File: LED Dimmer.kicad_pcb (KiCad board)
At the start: 2 copper layers, 118.1 x 74.9 mm, 82 parts, among them P1 Red Load, P2 Green Load, P3 Blue Load, P4 PWR, Q1 TIP31C, Q2 TIP31C, Q3 TIP31C, Q4 Q_PNP_EBC, Q5 Q_PNP_EBC, Q6 Q_NPN_EBC, SW1 SW_SPDT, SW10 SW_SPDT, SW11 SW_SPDT, SW12 SW_SPDT, SW2 SW_SPDT, SW3 SW_SPDT, SW4 SW_SPDT, SW5 SW_SPDT, SW6 SW_SPDT, SW7 SW_SPDT, SW8 SW_SPDT, SW9 SW_SPDT, U1 LM358, U2 LM358, U3 LM358, U4 LM555N

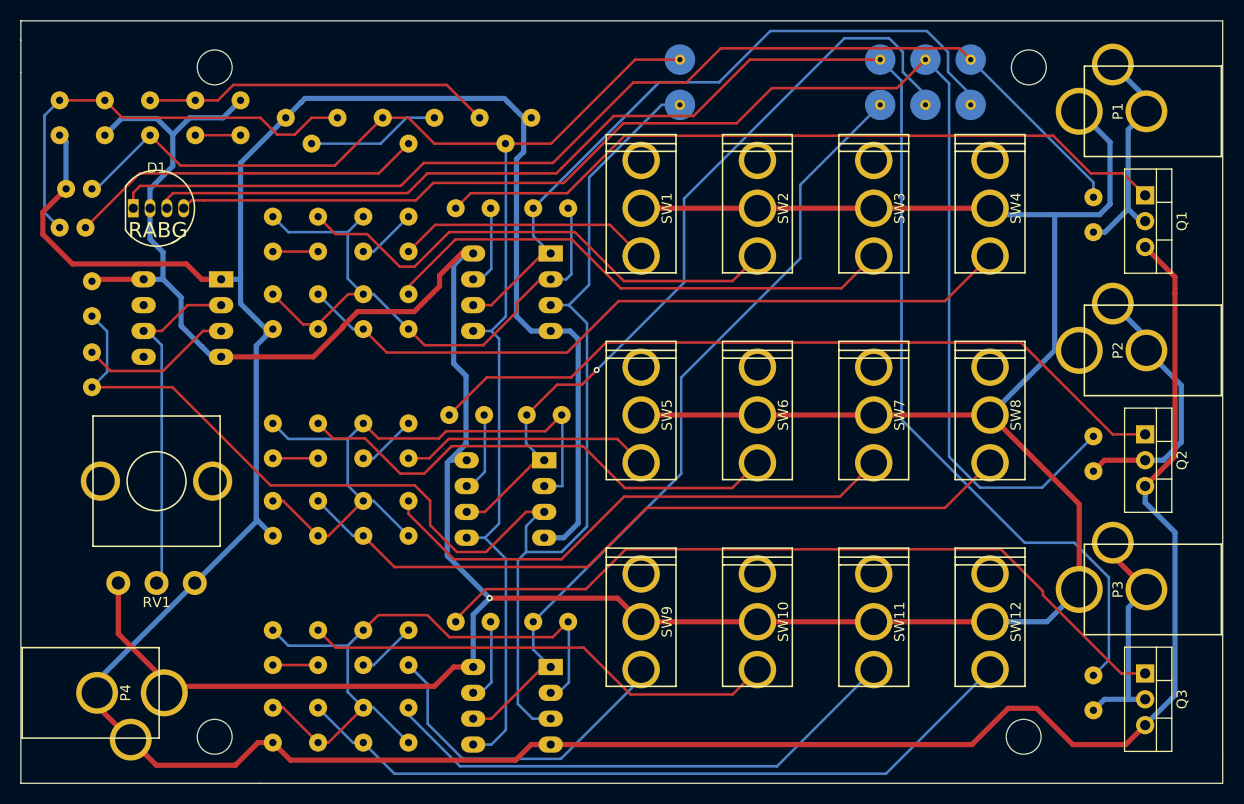
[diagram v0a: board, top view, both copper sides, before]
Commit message: Copper pour, maybe
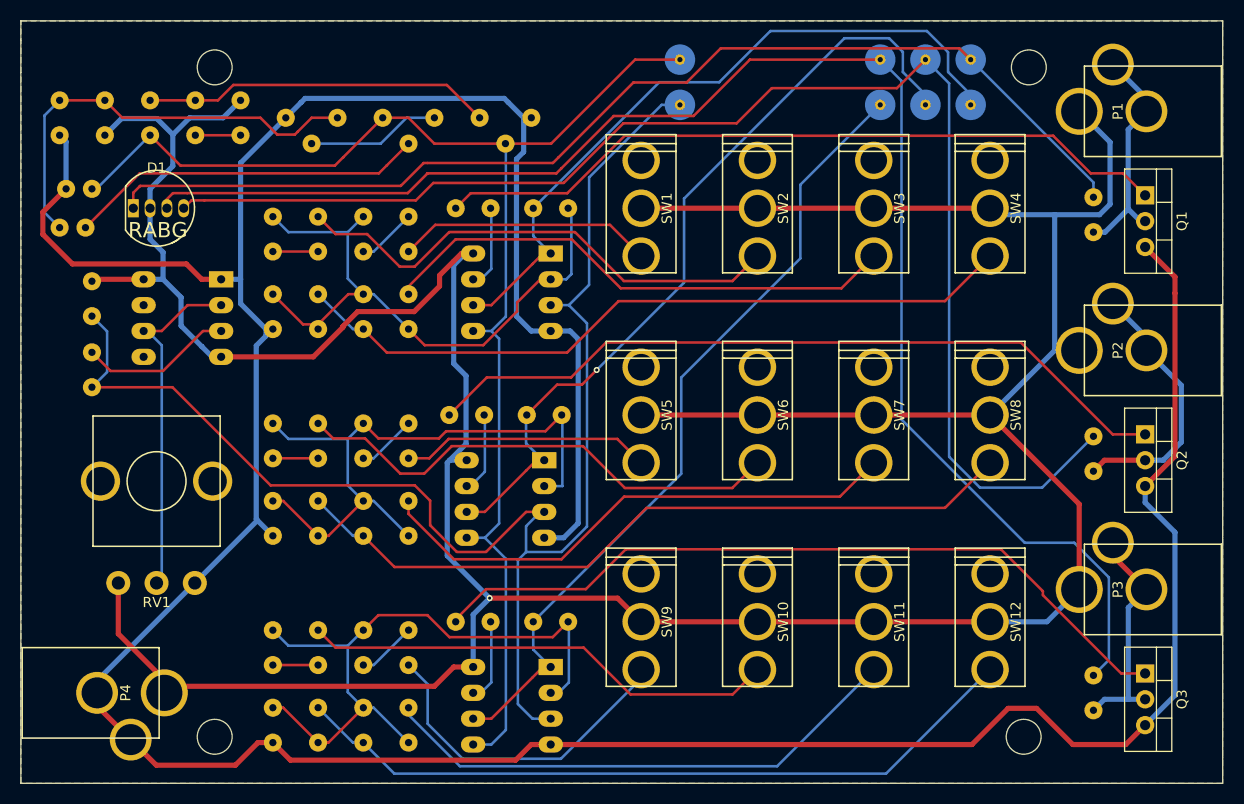
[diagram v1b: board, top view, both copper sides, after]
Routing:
- added copper zone on B.Cu, net GND
- added copper zone on F.Cu, net GND
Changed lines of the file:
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@@
     (links 144)
     (no_connects 0)
-    (area 87.007699 46.5678 206.362301 121.970001)
+    (area 87.007699 46.5678 206.362301 138.2302)
     (thickness 1.6)
     (drawings 17)
@@
     (visible_elements 7FFFFFFF)
     (pcbplotparams
-      (layerselection 0x00030_80000001)
+      (layerselection 0x010f0_80000001)
       (usegerberextensions false)
       (excludeedgelayer true)
@@
       (outputformat 1)
       (mirror false)
-      (drillshape 1)
+      (drillshape 0)
       (scaleselection 1)
-      (outputdirectory ""))
+      (outputdirectory Gerbs/))
   )
   (net 0 "")
@@
   (segment (start 101.4795 101.7205) (end 100.965 102.235) (width 0.254) (layer B.Cu) (net 47))
   (segment (start 101.4795 78.8735) (end 101.4795 101.7205) (width 0.254) (layer B.Cu) (net 47))
+  (zone (net 2) (net_name GND) (layer F.Cu) (hatch edge 0.508)
+    (connect_pads (clearance 0.508))
+    (min_thickness 0.254)
+    (fill (arc_segments 16) (thermal_gap 0.508) (thermal_bridge_width 0.508))
+    (polygon
+      (pts
+        (xy 205.74 121.92) (xy 87.63 121.92) (xy 87.63 46.99) (xy 205.74 46.99)
+      )
+    )
+  )
+  (zone (net 2) (net_name GND) (layer B.Cu) (hatch edge 0.508)
+    (connect_pads (clearance 0.508))
+    (min_thickness 0.254)
+    (fill (arc_segments 16) (thermal_gap 0.508) (thermal_bridge_width 0.508))
+    (polygon
+      (pts
+        (xy 205.74 121.92) (xy 87.63 121.92) (xy 87.63 46.99) (xy 205.74 46.99)
+      )
+    )
+  )
 )
